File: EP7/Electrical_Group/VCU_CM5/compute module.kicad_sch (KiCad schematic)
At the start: 5 parts

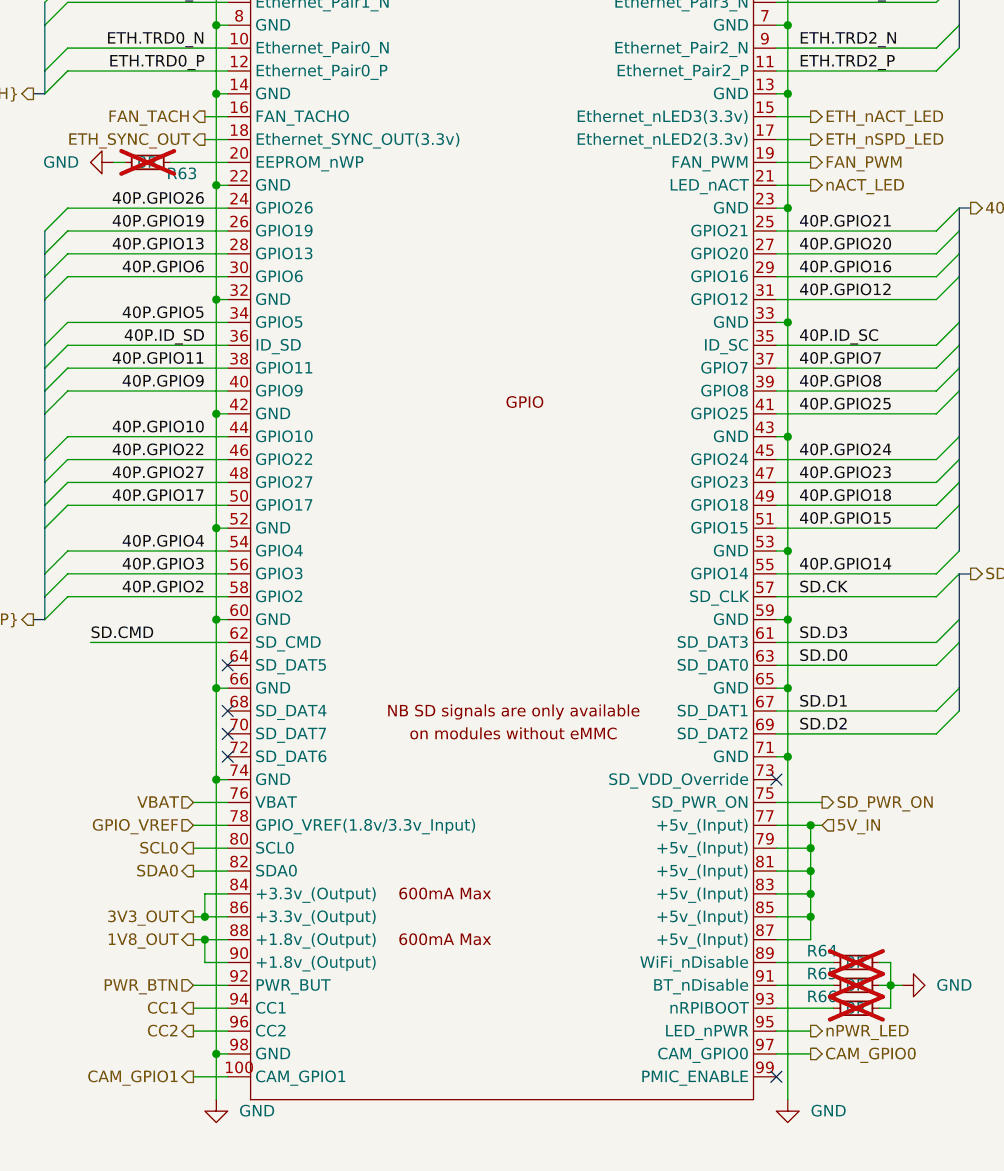
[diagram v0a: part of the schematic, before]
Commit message: VCU_CM5 initial floorplan
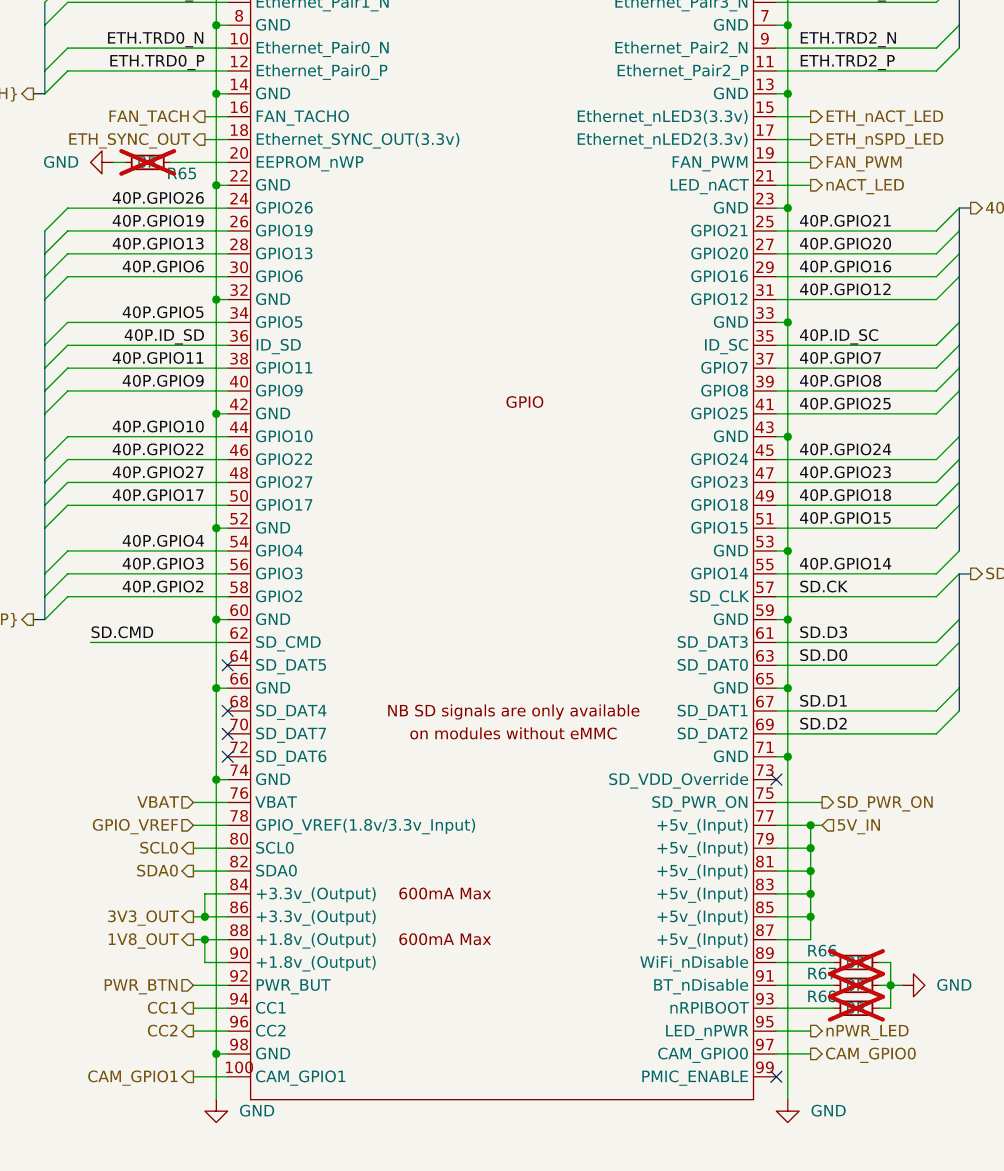
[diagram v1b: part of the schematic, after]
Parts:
- renumbered R63 to R65, R64 to R66, R65 to R67, R66 to R68
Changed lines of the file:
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@@
 		(dnp no)
 		(fields_autoplaced yes)
-		(property "Reference" "#PWR0126"
+		(property "Reference" "#PWR0129"
 			(at 33.02 49.53 0)
 			(effects
@@
 			(project "VCU"
 				(path "/eb296f24-894e-4ea0-b0cd-3ba211155378/0b024046-a452-472c-8933-8dd8af0d7b70/0fe8afc8-b7c5-49f3-8318-2bf5095c7824"
-					(reference "#PWR0126")
+					(reference "#PWR0129")
 					(unit 1)
 				)
@@
 		(dnp no)
 		(fields_autoplaced yes)
-		(property "Reference" "#PWR0129"
+		(property "Reference" "#PWR0132"
 			(at 133.35 140.97 0)
 			(effects
@@
 			(project "VCU"
 				(path "/eb296f24-894e-4ea0-b0cd-3ba211155378/0b024046-a452-472c-8933-8dd8af0d7b70/0fe8afc8-b7c5-49f3-8318-2bf5095c7824"
-					(reference "#PWR0129")
+					(reference "#PWR0132")
 					(unit 1)
 				)
@@
 		(on_board yes)
 		(dnp yes)
-		(property "Reference" "R64"
+		(property "Reference" "R66"
 			(at 118.11 137.16 90)
 			(effects
@@
 			(project "VCU"
 				(path "/eb296f24-894e-4ea0-b0cd-3ba211155378/0b024046-a452-472c-8933-8dd8af0d7b70/0fe8afc8-b7c5-49f3-8318-2bf5095c7824"
-					(reference "R64")
+					(reference "R66")
 					(unit 1)
 				)
@@
 		(on_board yes)
 		(dnp yes)
-		(property "Reference" "R63"
+		(property "Reference" "R65"
 			(at 46.99 50.8 90)
 			(effects
@@
 			(project "VCU"
 				(path "/eb296f24-894e-4ea0-b0cd-3ba211155378/0b024046-a452-472c-8933-8dd8af0d7b70/0fe8afc8-b7c5-49f3-8318-2bf5095c7824"
-					(reference "R63")
+					(reference "R65")
 					(unit 1)
 				)
@@
 		(on_board yes)
 		(dnp yes)
-		(property "Reference" "R65"
+		(property "Reference" "R67"
 			(at 118.11 139.7 90)
 			(effects
@@
 			(project "VCU"
 				(path "/eb296f24-894e-4ea0-b0cd-3ba211155378/0b024046-a452-472c-8933-8dd8af0d7b70/0fe8afc8-b7c5-49f3-8318-2bf5095c7824"
-					(reference "R65")
+					(reference "R67")
 					(unit 1)
 				)
@@
 		(dnp no)
 		(fields_autoplaced yes)
-		(property "Reference" "#PWR0131"
+		(property "Reference" "#PWR0134"
 			(at 247.65 160.02 0)
 			(effects
@@
 			(project "VCU"
 				(path "/eb296f24-894e-4ea0-b0cd-3ba211155378/0b024046-a452-472c-8933-8dd8af0d7b70/0fe8afc8-b7c5-49f3-8318-2bf5095c7824"
-					(reference "#PWR0131")
+					(reference "#PWR0134")
 					(unit 1)
 				)
@@
 		(on_board yes)
 		(dnp yes)
-		(property "Reference" "R66"
+		(property "Reference" "R68"
 			(at 118.11 142.24 90)
 			(effects
@@
 			(project "VCU"
 				(path "/eb296f24-894e-4ea0-b0cd-3ba211155378/0b024046-a452-472c-8933-8dd8af0d7b70/0fe8afc8-b7c5-49f3-8318-2bf5095c7824"
-					(reference "R66")
+					(reference "R68")
 					(unit 1)
 				)
@@
 		(dnp no)
 		(fields_autoplaced yes)
-		(property "Reference" "#PWR0130"
+		(property "Reference" "#PWR0133"
 			(at 184.15 160.02 0)
 			(effects
@@
 			(project "VCU"
 				(path "/eb296f24-894e-4ea0-b0cd-3ba211155378/0b024046-a452-472c-8933-8dd8af0d7b70/0fe8afc8-b7c5-49f3-8318-2bf5095c7824"
-					(reference "#PWR0130")
+					(reference "#PWR0133")
 					(unit 1)
 				)
@@
 		(dnp no)
 		(fields_autoplaced yes)
-		(property "Reference" "#PWR0127"
+		(property "Reference" "#PWR0130"
 			(at 50.8 160.02 0)
 			(effects
@@
 			(project "VCU"
 				(path "/eb296f24-894e-4ea0-b0cd-3ba211155378/0b024046-a452-472c-8933-8dd8af0d7b70/0fe8afc8-b7c5-49f3-8318-2bf5095c7824"
-					(reference "#PWR0127")
+					(reference "#PWR0130")
 					(unit 1)
 				)
@@
 		(dnp no)
 		(fields_autoplaced yes)
-		(property "Reference" "#PWR0128"
+		(property "Reference" "#PWR0131"
 			(at 114.3 160.02 0)
 			(effects
@@
 			(project "VCU"
 				(path "/eb296f24-894e-4ea0-b0cd-3ba211155378/0b024046-a452-472c-8933-8dd8af0d7b70/0fe8afc8-b7c5-49f3-8318-2bf5095c7824"
-					(reference "#PWR0128")
+					(reference "#PWR0131")
 					(unit 1)
 				)
